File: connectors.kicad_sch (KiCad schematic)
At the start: 4 parts, among them J1 Conn_01x04_Pin, J2 Conn_01x04_Pin, J3 Conn_02x03_Odd_Even, J4 Conn_01x09_Pin

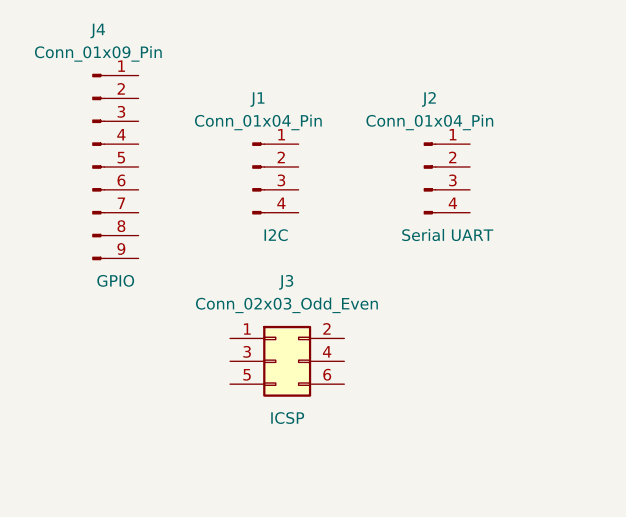
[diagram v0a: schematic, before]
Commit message: Wiring done
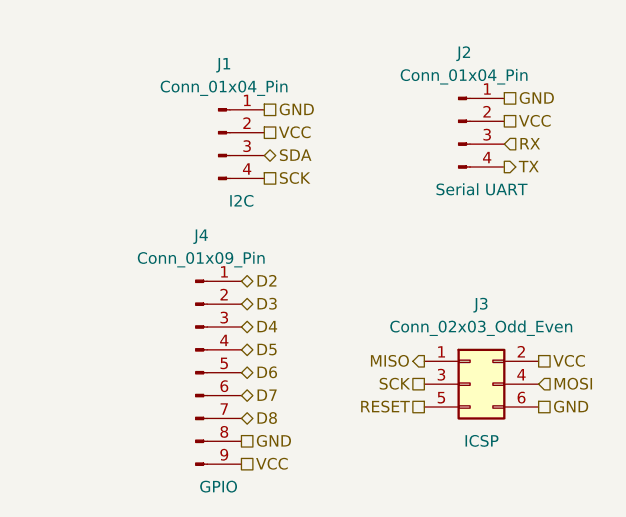
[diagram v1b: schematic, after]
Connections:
- net GND: now reaches J2.1 (Pin_1)
- net GND: now also J1.1 (Pin_1), J3.6 (Pin_6), J4.8 (Pin_8)
- net VCC: now reaches J2.2 (Pin_2)
- net VCC: now also J1.2 (Pin_2), J3.2 (Pin_2), J4.9 (Pin_9)
- net RX: now reaches J2.3 (Pin_3)
- net TX: now reaches J2.4 (Pin_4)
- net MISO: now reaches J3.1 (Pin_1)
- net SCK: now reaches J3.3 (Pin_3)
- net SCK: now also J1.4 (Pin_4)
- net MOSI: now reaches J3.4 (Pin_4)
- net RESET: now reaches J3.5 (Pin_5)
- net SDA: now reaches J1.3 (Pin_3)
- net D2: now reaches J4.1 (Pin_1)
- net D3: now reaches J4.2 (Pin_2)
- net D4: now reaches J4.3 (Pin_3)
- net D5: now reaches J4.4 (Pin_4)
- net D6: now reaches J4.5 (Pin_5)
- net D7: now reaches J4.6 (Pin_6)
- net D8: now reaches J4.7 (Pin_7)
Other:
- moved on the sheet: J1, J2, J3, J4
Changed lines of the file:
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@@
 (kicad_sch (version 20230121) (generator eeschema)
   (paper "A4")
-  (symbol (lib_id "Connector:Conn_01x04_Pin") (at 69.85 50.8 0) (unit 1)
+  (hierarchical_label "GND" (shape passive) (at 52.07 44.45 0) (fields_autoplaced)
+    (effects (font (size 1.27 1.27)) (justify left))
+  )
+  (hierarchical_label "SCK" (shape passive) (at 52.07 52.07 0) (fields_autoplaced)
+    (effects (font (size 1.27 1.27)) (justify left))
+  )
+  (hierarchical_label "MISO" (shape output) (at 69.85 72.39 180) (fields_autoplaced)
+    (effects (font (size 1.27 1.27)) (justify right))
+  )
+  (hierarchical_label "D3" (shape bidirectional) (at 49.53 66.04 0) (fields_autoplaced)
+    (effects (font (size 1.27 1.27)) (justify left))
+  )
+  (hierarchical_label "D7" (shape bidirectional) (at 49.53 76.2 0) (fields_autoplaced)
+    (effects (font (size 1.27 1.27)) (justify left))
+  )
+  (hierarchical_label "MOSI" (shape input) (at 82.55 74.93 0) (fields_autoplaced)
+    (effects (font (size 1.27 1.27)) (justify left))
+  )
+  (hierarchical_label "TX" (shape output) (at 78.74 50.8 0) (fields_autoplaced)
+    (effects (font (size 1.27 1.27)) (justify left))
+  )
+  (hierarchical_label "GND" (shape passive) (at 82.55 77.47 0) (fields_autoplaced)
+    (effects (font (size 1.27 1.27)) (justify left))
+  )
+  (hierarchical_label "SDA" (shape bidirectional) (at 52.07 49.53 0) (fields_autoplaced)
+    (effects (font (size 1.27 1.27)) (justify left))
+  )
+  (hierarchical_label "D4" (shape bidirectional) (at 49.53 68.58 0) (fields_autoplaced)
+    (effects (font (size 1.27 1.27)) (justify left))
+  )
+  (hierarchical_label "GND" (shape passive) (at 78.74 43.18 0) (fields_autoplaced)
+    (effects (font (size 1.27 1.27)) (justify left))
+  )
+  (hierarchical_label "VCC" (shape passive) (at 52.07 46.99 0) (fields_autoplaced)
+    (effects (font (size 1.27 1.27)) (justify left))
+  )
+  (hierarchical_label "D5" (shape bidirectional) (at 49.53 71.12 0) (fields_autoplaced)
+    (effects (font (size 1.27 1.27)) (justify left))
+  )
+  (hierarchical_label "D8" (shape bidirectional) (at 49.53 78.74 0) (fields_autoplaced)
+    (effects (font (size 1.27 1.27)) (justify left))
+  )
+  (hierarchical_label "VCC" (shape passive) (at 78.74 45.72 0) (fields_autoplaced)
+    (effects (font (size 1.27 1.27)) (justify left))
+  )
+  (hierarchical_label "GND" (shape passive) (at 49.53 81.28 0) (fields_autoplaced)
+    (effects (font (size 1.27 1.27)) (justify left))
+  )
+  (hierarchical_label "VCC" (shape passive) (at 49.53 83.82 0) (fields_autoplaced)
+    (effects (font (size 1.27 1.27)) (justify left))
+  )
+  (hierarchical_label "SCK" (shape passive) (at 69.85 74.93 180) (fields_autoplaced)
+    (effects (font (size 1.27 1.27)) (justify right))
+  )
+  (hierarchical_label "VCC" (shape passive) (at 82.55 72.39 0) (fields_autoplaced)
+    (effects (font (size 1.27 1.27)) (justify left))
+  )
+  (hierarchical_label "RX" (shape input) (at 78.74 48.26 0) (fields_autoplaced)
+    (effects (font (size 1.27 1.27)) (justify left))
+  )
+  (hierarchical_label "RESET" (shape passive) (at 69.85 77.47 180) (fields_autoplaced)
+    (effects (font (size 1.27 1.27)) (justify right))
+  )
+  (hierarchical_label "D2" (shape bidirectional) (at 49.53 63.5 0) (fields_autoplaced)
+    (effects (font (size 1.27 1.27)) (justify left))
+  )
+  (hierarchical_label "D6" (shape bidirectional) (at 49.53 73.66 0) (fields_autoplaced)
+    (effects (font (size 1.27 1.27)) (justify left))
+  )
+  (symbol (lib_id "Connector:Conn_01x04_Pin") (at 73.66 45.72 0) (unit 1)
     (in_bom yes) (on_board yes) (dnp no)
-    (property "Reference" "J2" (at 70.485 43.18 0)
+    (property "Reference" "J2" (at 74.295 38.1 0)
       (effects (font (size 1.27 1.27)))
     )
-    (property "Value" "Conn_01x04_Pin" (at 70.485 45.72 0)
+    (property "Value" "Conn_01x04_Pin" (at 74.295 40.64 0)
       (effects (font (size 1.27 1.27)))
     )
-    (property "Footprint" "Connector_PinHeader_2.54mm:PinHeader_1x04_P2.54mm_Vertical" (at 69.85 50.8 0)
+    (property "Footprint" "Connector_PinHeader_2.54mm:PinHeader_1x04_P2.54mm_Vertical" (at 73.66 45.72 0)
       (effects (font (size 1.27 1.27)) hide)
     )
-    (property "Datasheet" "~" (at 69.85 50.8 0)
+    (property "Datasheet" "~" (at 73.66 45.72 0)
       (effects (font (size 1.27 1.27)) hide)
     )
-    (property "Purpose" "Serial UART" (at 72.39 58.42 0)
+    (property "Purpose" "Serial UART" (at 76.2 53.34 0)
       (effects (font (size 1.27 1.27)))
     )
@@
     )
   )
-  (symbol (lib_id "Connector_Generic:Conn_02x03_Odd_Even") (at 53.34 72.39 0) (unit 1)
+  (symbol (lib_id "Connector_Generic:Conn_02x03_Odd_Even") (at 74.93 74.93 0) (unit 1)
     (in_bom yes) (on_board yes) (dnp no)
-    (property "Reference" "J3" (at 54.61 63.5 0)
+    (property "Reference" "J3" (at 76.2 66.04 0)
       (effects (font (size 1.27 1.27)))
     )
-    (property "Value" "Conn_02x03_Odd_Even" (at 54.61 66.04 0)
+    (property "Value" "Conn_02x03_Odd_Even" (at 76.2 68.58 0)
       (effects (font (size 1.27 1.27)))
     )
-    (property "Footprint" "Connector_PinHeader_2.54mm:PinHeader_2x03_P2.54mm_Vertical" (at 53.34 72.39 0)
+    (property "Footprint" "Connector_PinHeader_2.54mm:PinHeader_2x03_P2.54mm_Vertical" (at 74.93 74.93 0)
       (effects (font (size 1.27 1.27)) hide)
     )
-    (property "Datasheet" "~" (at 53.34 72.39 0)
+    (property "Datasheet" "~" (at 74.93 74.93 0)
       (effects (font (size 1.27 1.27)) hide)
     )
-    (property "Purpose" "ICSP" (at 54.61 78.74 0)
+    (property "Purpose" "ICSP" (at 76.2 81.28 0)
       (effects (font (size 1.27 1.27)))
     )
@@
     )
   )
-  (symbol (lib_id "Connector:Conn_01x04_Pin") (at 50.8 50.8 0) (unit 1)
+  (symbol (lib_id "Connector:Conn_01x04_Pin") (at 46.99 46.99 0) (unit 1)
     (in_bom yes) (on_board yes) (dnp no)
-    (property "Reference" "J1" (at 51.435 43.18 0)
+    (property "Reference" "J1" (at 47.625 39.37 0)
       (effects (font (size 1.27 1.27)))
     )
-    (property "Value" "Conn_01x04_Pin" (at 51.435 45.72 0)
+    (property "Value" "Conn_01x04_Pin" (at 47.625 41.91 0)
       (effects (font (size 1.27 1.27)))
     )
-    (property "Footprint" "Connector_PinHeader_2.54mm:PinHeader_1x04_P2.54mm_Vertical" (at 50.8 50.8 0)
+    (property "Footprint" "Connector_PinHeader_2.54mm:PinHeader_1x04_P2.54mm_Vertical" (at 46.99 46.99 0)
       (effects (font (size 1.27 1.27)) hide)
     )
-    (property "Datasheet" "~" (at 50.8 50.8 0)
+    (property "Datasheet" "~" (at 46.99 46.99 0)
       (effects (font (size 1.27 1.27)) hide)
     )
-    (property "Purpose" "I2C" (at 53.34 58.42 0)
+    (property "Purpose" "I2C" (at 49.53 54.61 0)
       (effects (font (size 1.27 1.27)))
     )
@@
     )
   )
-  (symbol (lib_id "Connector:Conn_01x09_Pin") (at 33.02 50.8 0) (unit 1)
+  (symbol (lib_id "Connector:Conn_01x09_Pin") (at 44.45 73.66 0) (unit 1)
     (in_bom yes) (on_board yes) (dnp no)
-    (property "Reference" "J4" (at 33.655 35.56 0)
+    (property "Reference" "J4" (at 45.085 58.42 0)
       (effects (font (size 1.27 1.27)))
     )
-    (property "Value" "Conn_01x09_Pin" (at 33.655 38.1 0)
+    (property "Value" "Conn_01x09_Pin" (at 45.085 60.96 0)
       (effects (font (size 1.27 1.27)))
     )
-    (property "Footprint" "Connector_PinHeader_2.54mm:PinHeader_1x09_P2.54mm_Vertical" (at 33.02 50.8 0)
+    (property "Footprint" "Connector_PinHeader_2.54mm:PinHeader_1x09_P2.54mm_Vertical" (at 44.45 73.66 0)
       (effects (font (size 1.27 1.27)) hide)
     )
-    (property "Datasheet" "~" (at 33.02 50.8 0)
+    (property "Datasheet" "~" (at 44.45 73.66 0)
       (effects (font (size 1.27 1.27)) hide)
     )
-    (property "Purpose" "GPIO" (at 35.56 63.5 0)
+    (property "Purpose" "GPIO" (at 46.99 86.36 0)
       (effects (font (size 1.27 1.27)))
     )
